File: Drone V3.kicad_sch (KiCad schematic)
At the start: 2 parts, among them J1 Pad Terminals, U5 STM32F427ZGTx

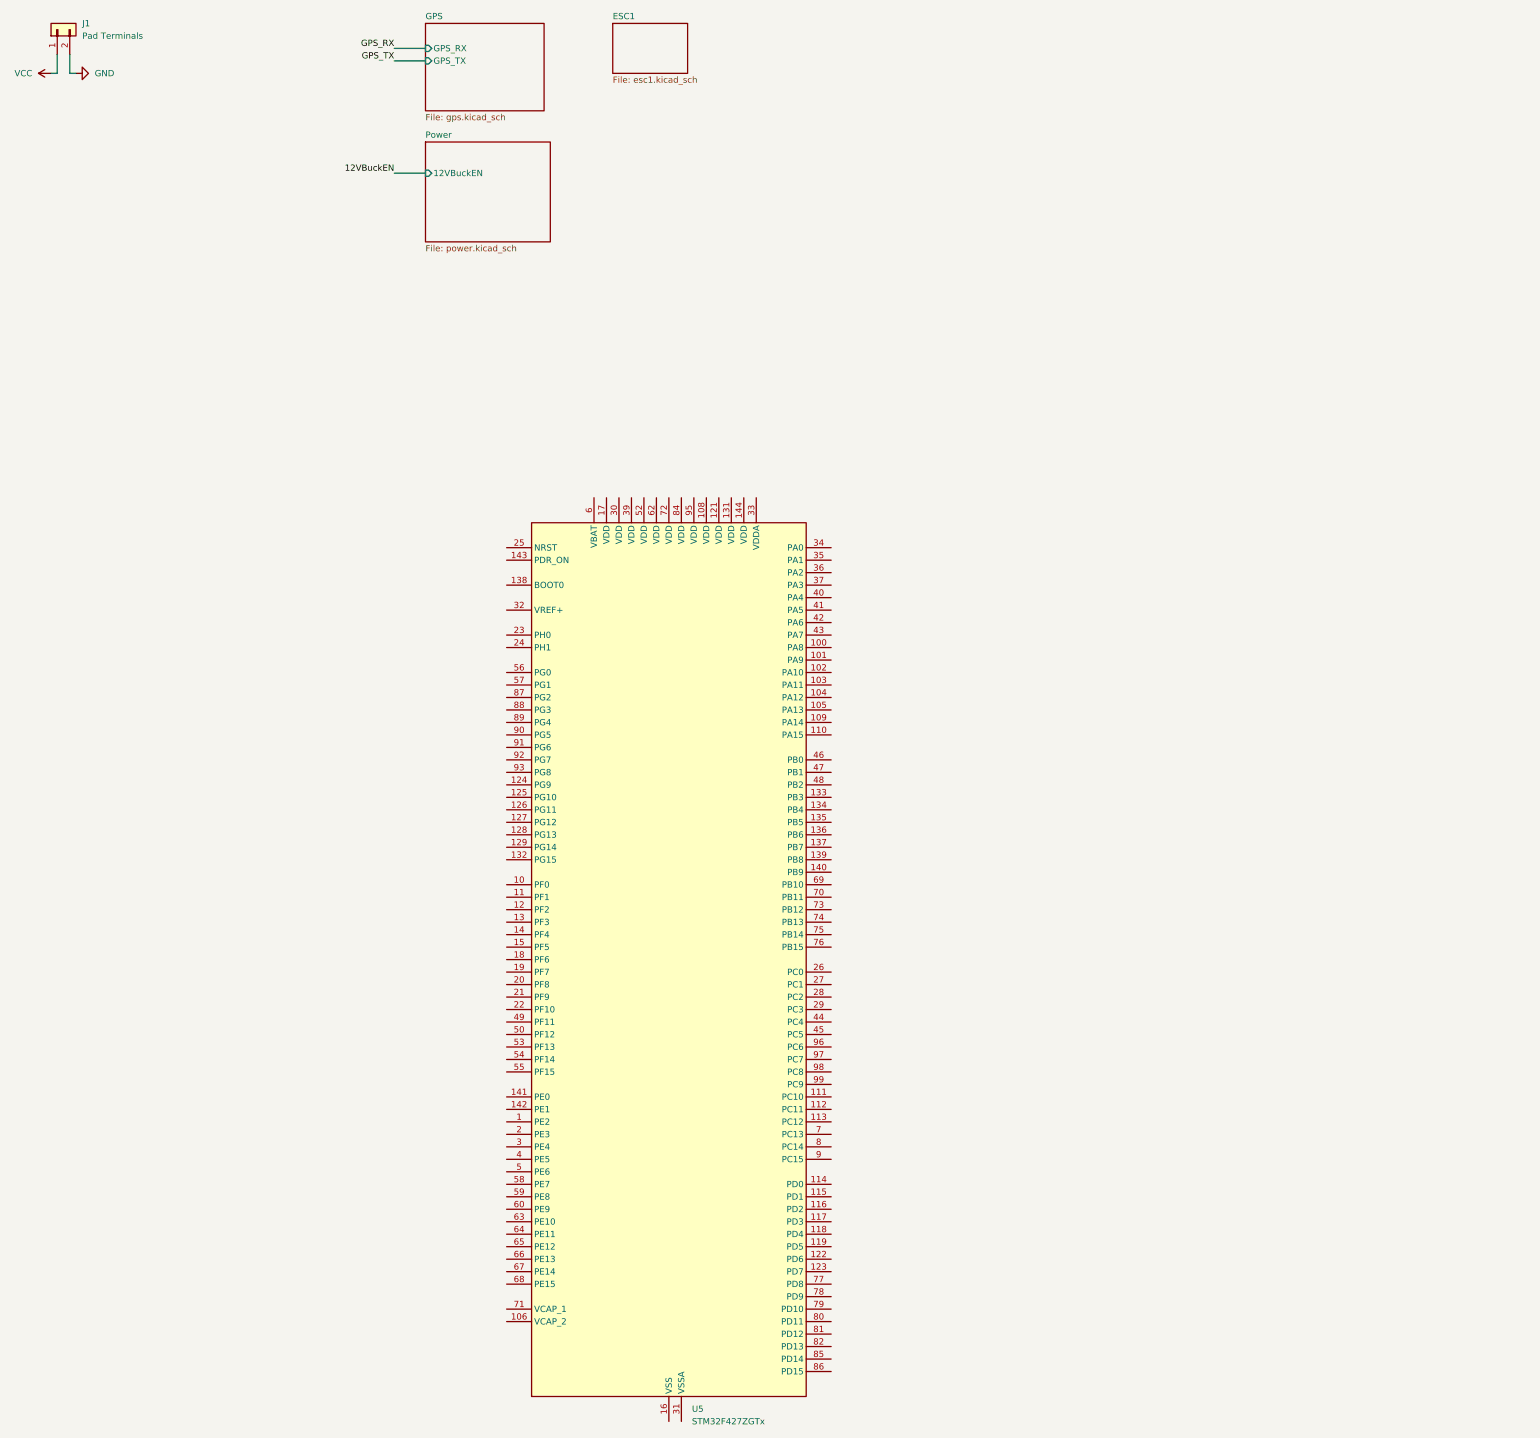
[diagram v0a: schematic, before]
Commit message: Drone PCB Update
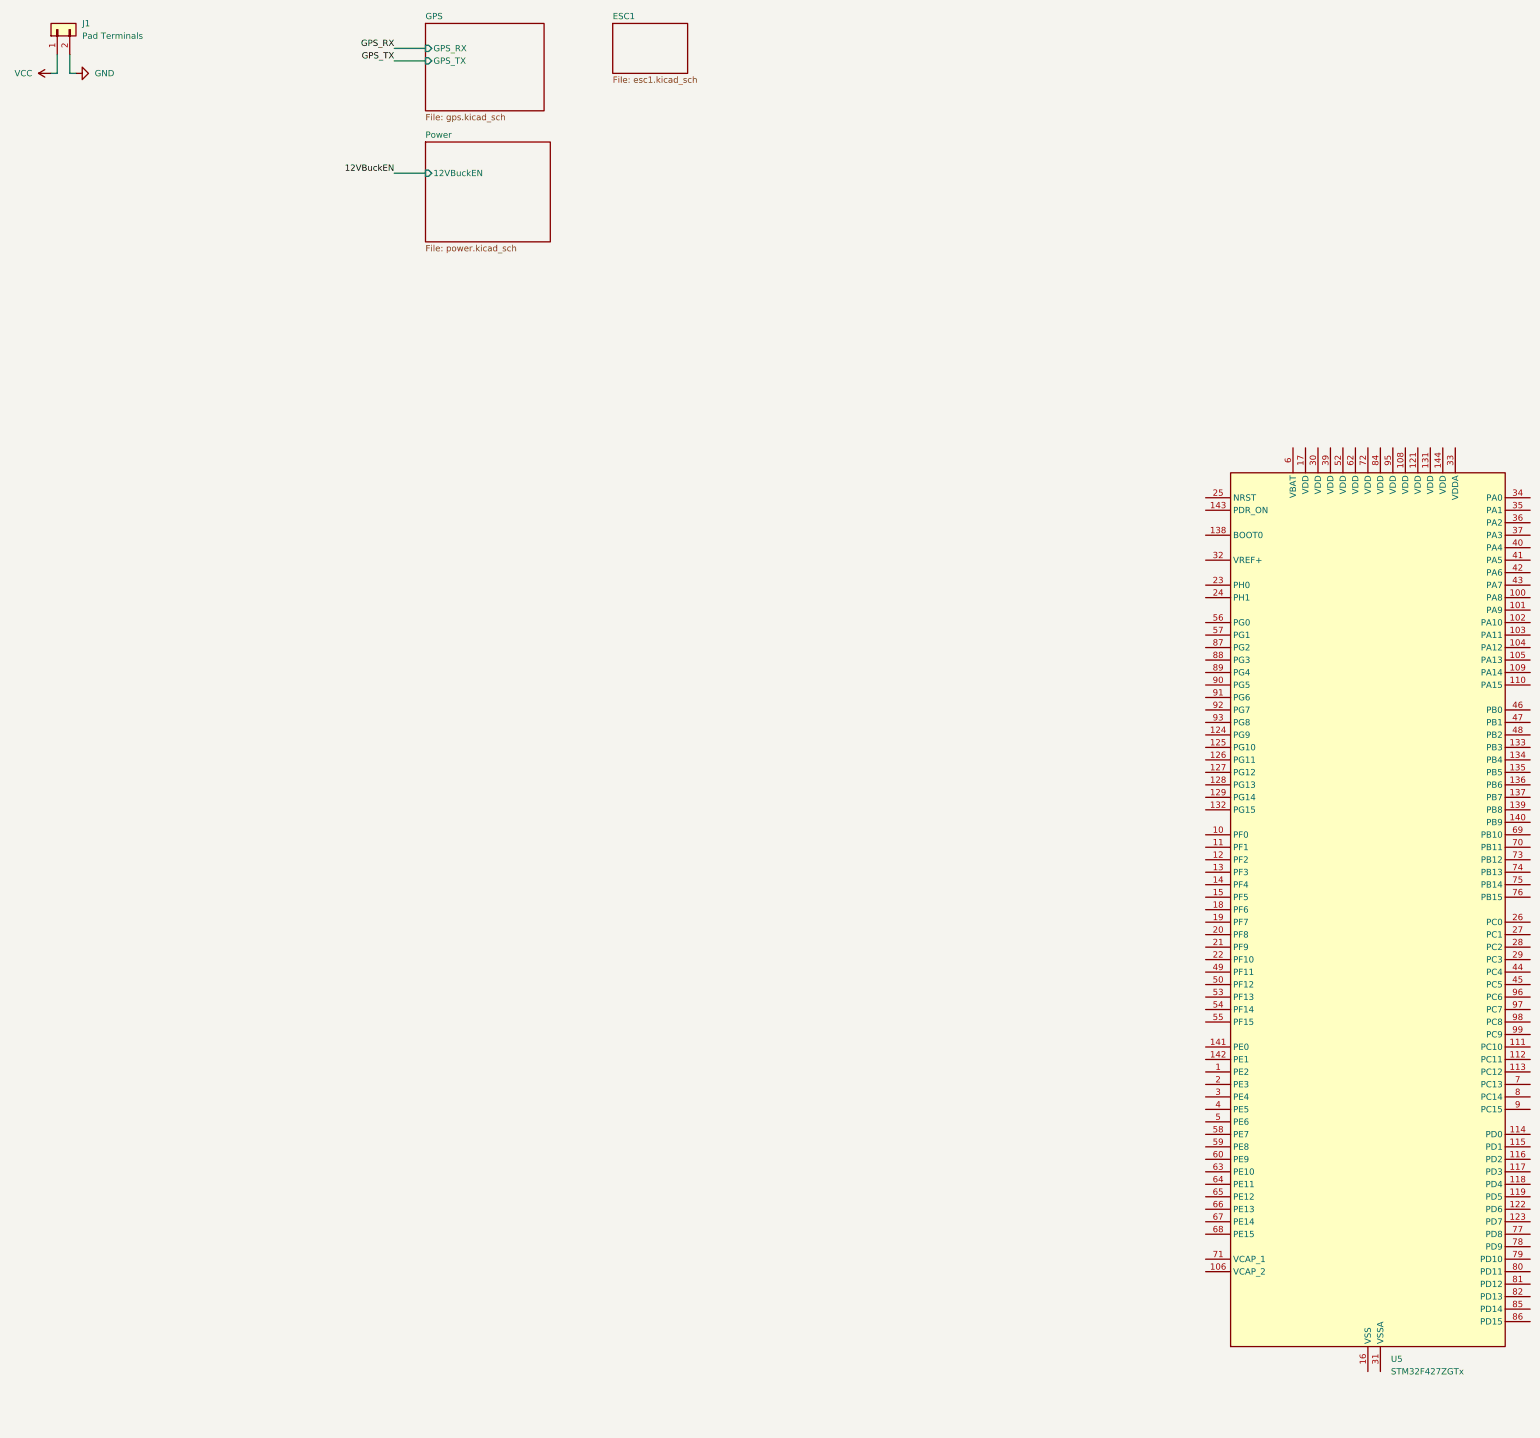
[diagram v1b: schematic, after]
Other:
- moved on the sheet: U5
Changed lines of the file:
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@@
 	(symbol
 		(lib_id "MCU_ST_STM32F4:STM32F427ZGTx")
-		(at 152.4 210.82 0)
+		(at 294.64 200.66 0)
 		(unit 1)
 		(exclude_from_sim no)
@@
 		(fields_autoplaced yes)
 		(property "Reference" "U5"
-			(at 157.0833 302.26 0)
+			(at 299.3233 292.1 0)
 			(effects
 				(font
@@
 		)
 		(property "Value" "STM32F427ZGTx"
-			(at 157.0833 304.8 0)
+			(at 299.3233 294.64 0)
 			(effects
 				(font
@@
 		)
 		(property "Footprint" "Package_QFP:LQFP-144_20x20mm_P0.5mm"
-			(at 124.46 299.72 0)
+			(at 266.7 289.56 0)
 			(effects
 				(font
@@
 		)
 		(property "Datasheet" "https://www.st.com/resource/en/datasheet/stm32f427zg.pdf"
-			(at 152.4 210.82 0)
+			(at 294.64 200.66 0)
 			(effects
 				(font
@@
 		)
 		(property "Description" "STMicroelectronics Arm Cortex-M4 MCU, 1024KB flash, 256KB RAM, 180 MHz, 1.7-3.6V, 114 GPIO, LQFP144"
-			(at 152.4 210.82 0)
+			(at 294.64 200.66 0)
 			(effects
 				(font
